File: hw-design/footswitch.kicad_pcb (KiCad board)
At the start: 2 copper layers, 248.9 x 74.2 mm, 101 parts, among them CN1 CONN_PANNEL_2X2, CN2 CONN_PANNEL_2X2, J1 RJ45_CHAIN_MAIN, J2 RJ45_CHAIN_EXTENSION, P1 HEADER_5X2, P2 HEADER_5X2, P3 CONN_8X2, P4 CONN_8X2, Q1 MMBT3904, Q2 MMBT3906, Q3 MMBT3904, U1 LPC111X_LQFP48, U2 MC7805, U3 NCP1117DT33G, U4 MAX13450E, U5 74HC245, U6 74HC245, X1 10MHz

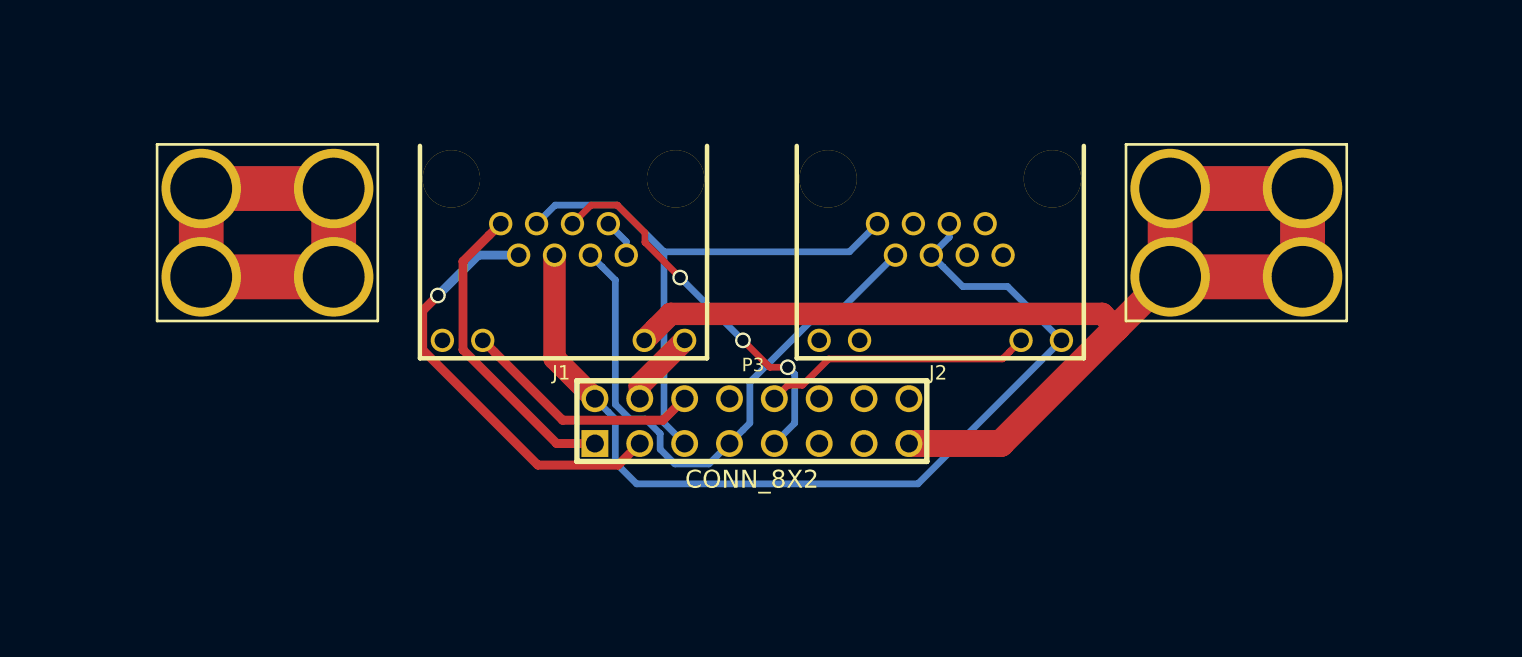
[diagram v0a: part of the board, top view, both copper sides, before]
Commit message: wip: tracing signals and adding a ground plane to the mini-pcb with connectors
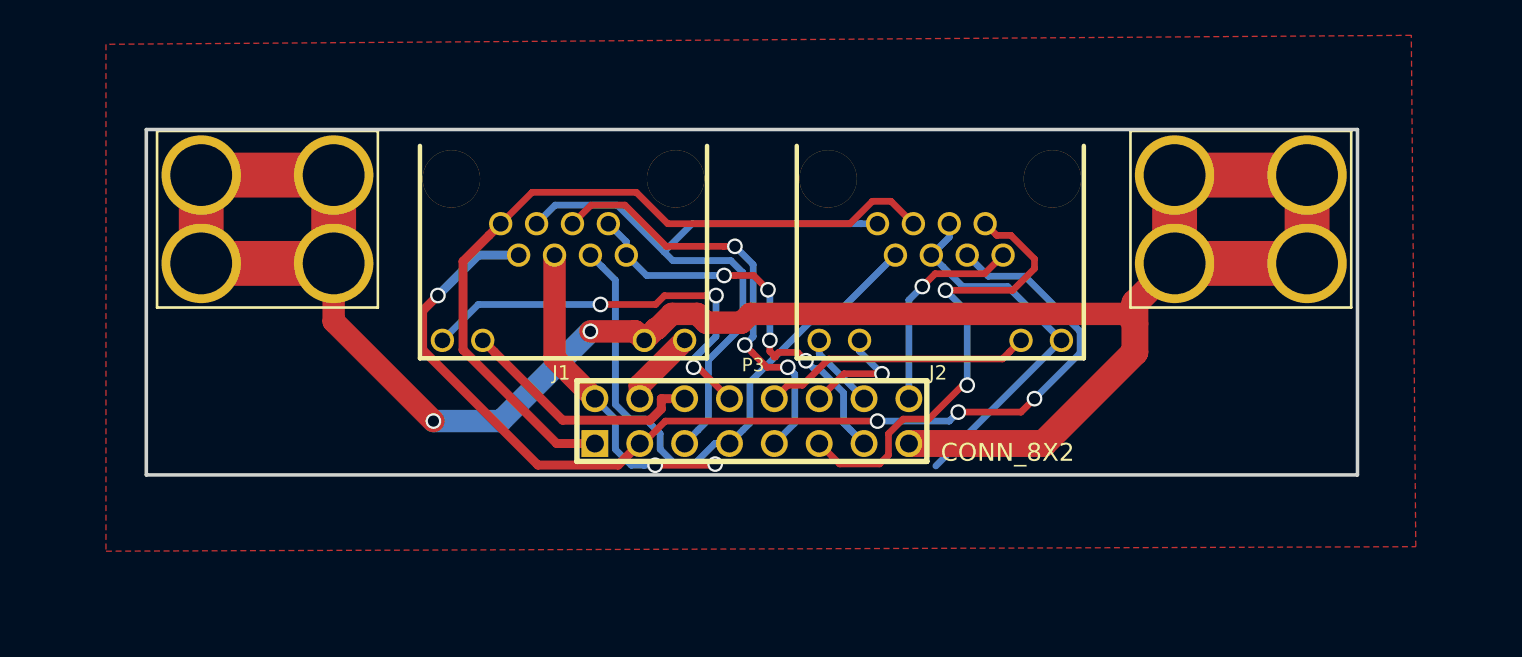
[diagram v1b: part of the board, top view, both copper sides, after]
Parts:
- moved CN1 0.80 mm to (251.2, 176.0)
- moved CN2 0.76 mm to (196.1, 176.0)
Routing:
- net P3_RS422_TX-: track 24.5 -> 60.9 mm, vias 1 -> 4
- net P3_DGND: track 101.3 -> 130.3 mm, vias 0 -> 2
- net P3_GND_FB: track 0.00 -> 27.0 mm, vias 0 -> 2
- net P3_RS422_TX+: track 17.7 -> 43.6 mm
- net P3_MAIN_LED1A: track 0.00 -> 23.9 mm, vias 0 -> 3
- net P3_MAIN_LOAD: track 2.20 -> 23.4 mm, vias 0 -> 4
- net Net-(R12-Pad1): track 7.57 -> 23.6 mm, vias 0 -> 1
- net GND_FB: track 46.1 -> 30.1 mm, vias 2 -> 1
- net P3_VCC: track 53.9 -> 40.3 mm, vias 0 -> 2
- net P3_EXT_LOAD: track 0.00 -> 12.0 mm, vias 0 -> 1
- net DGND: track 179.8 -> 170.0 mm, vias 59 -> 58
- net Net-(Q2-Pad1): track 3.66 -> 13.4 mm, vias 2 -> 3
- net P3_EXT_LED1C: track 0.00 -> 6.56 mm, vias 0 -> 1
- net P3_RS422_RX+: track 32.8 -> 37.5 mm
- net P3_EXT_LED1A: track 0.00 -> 4.35 mm
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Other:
- outline, holes or cut-outs redrawn
